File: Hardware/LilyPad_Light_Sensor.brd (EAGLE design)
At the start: 19.5 x 19.5 mm, 11 parts, among them U3 ALS-PT19

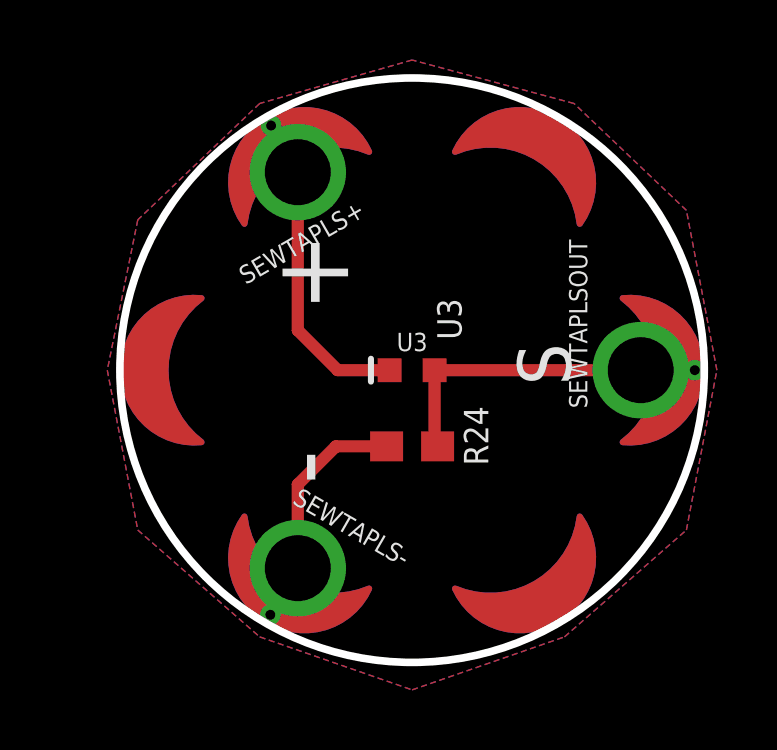
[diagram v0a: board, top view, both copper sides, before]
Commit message: Cleaned up some things
Read for review
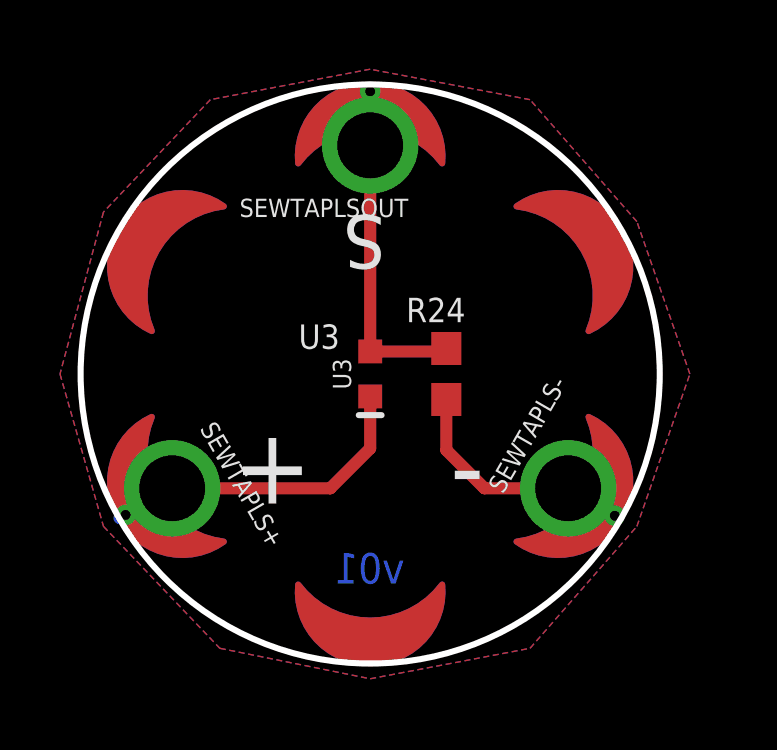
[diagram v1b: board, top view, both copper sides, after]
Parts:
- moved ST3 12.2 mm to (3.05, 13.5), turned to 240 degrees
- moved SEWTAPLSOUT 11.7 mm to (9.65, 17.3), turned to 180 degrees
- moved SEWTAPLS+ 11.3 mm to (3.05, 5.84), turned to 300 degrees
- moved ST2 10.4 mm to (16.3, 13.5), turned to 120 degrees
- moved ST1 9.94 mm to (9.65, 2.03), turned to 0 degrees
- moved SEWTAPLS- 9.40 mm to (16.3, 5.84), turned to 60 degrees
- moved R24 2.67 mm to (12.2, 9.65), turned to 90 degrees
- moved U3 1.40 mm to (9.65, 9.65), turned to 90 degrees
- moved U$5 1.15 mm to (9.65, 9.29), turned to 0 degrees
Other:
- board size 19.5 x 19.5 mm -> 19.3 x 19.3 mm
- board text added: "Inches"
- board text added: "v01"
